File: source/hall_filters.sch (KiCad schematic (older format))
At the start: 5 parts

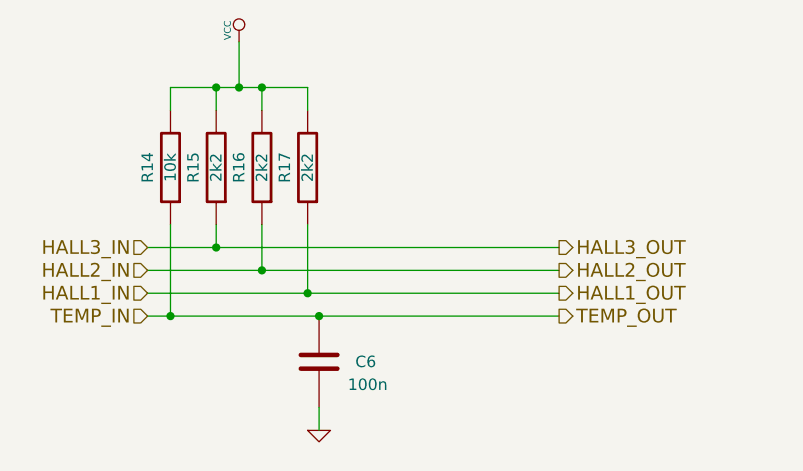
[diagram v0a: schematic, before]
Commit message: V1.0
V1.0
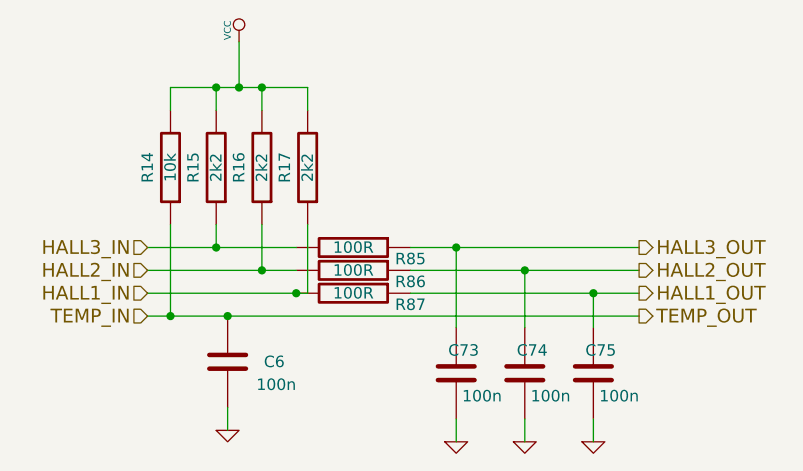
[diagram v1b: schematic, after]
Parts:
- added C73, C74, C75: 100n, Capacitor_SMD:C_0603_1608Metric, symbol BLDC_4-rescue:C-RESCUE-BLDC_4
- added R85, R86, R87: 100R, Resistor_SMD:R_0603_1608Metric, symbol BLDC_4-rescue:R-RESCUE-BLDC_4
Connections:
- net GND: now also C73.1, C74.1, C75.1
- net HALL1_IN: now also R87.2
- net HALL2_IN: now also R86.2
- net HALL3_IN: now also R85.2
- new net HALL1_OUT: C75.2, R87.1
- new net HALL2_OUT: C74.2, R86.1
- new net HALL3_OUT: C73.2, R85.1
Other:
- moved on the sheet: C6
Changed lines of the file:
@@
 Text HLabel 3500 3350 0    60   Input ~ 0
 TEMP_IN
-Text HLabel 5300 3050 2    60   Output ~ 0
+Text HLabel 5650 3050 2    60   Output ~ 0
 HALL3_OUT
-Text HLabel 5300 3150 2    60   Output ~ 0
+Text HLabel 5650 3150 2    60   Output ~ 0
 HALL2_OUT
-Text HLabel 5300 3250 2    60   Output ~ 0
+Text HLabel 5650 3250 2    60   Output ~ 0
 HALL1_OUT
-Text HLabel 5300 3350 2    60   Output ~ 0
+Text HLabel 5650 3350 2    60   Output ~ 0
 TEMP_OUT
 $Comp
 L BLDC_4-rescue:C-RESCUE-BLDC_4 C?
 U 1 1 5C7712C3
-P 4250 3550
+P 3850 3550
 AR Path="/5C7712C3" Ref="C?"  Part="1"
 AR Path="/53FBA77E/5C7712C3" Ref="C6"  Part="1"
-F 0 "C6" H 4000 3550 50  0000 L CNN
-F 1 "100n" H 3950 3650 50  0000 L CNN
-F 2 "Capacitor_SMD:C_0603_1608Metric" H 4250 3550 60  0001 C CNN
-F 3 "" H 4250 3550 60  0001 C CNN
-	1    4250 3550
-	-1   0    0    1
-$EndComp
-Wire Wire Line
-	4250 3350 5300 3350
+F 0 "C6" H 3600 3550 50  0000 L CNN
+F 1 "100n" H 3550 3650 50  0000 L CNN
+F 2 "Capacitor_SMD:C_0603_1608Metric" H 3850 3550 60  0001 C CNN
+F 3 "" H 3850 3550 60  0001 C CNN
+	1    3850 3550
+	-1   0    0    1
+$EndComp
 $Comp
 L BLDC_4-rescue:GND-RESCUE-BLDC_4 #PWR?
 U 1 1 5C7716C9
-P 4250 3850
+P 3850 3850
 AR Path="/504F83BE/5C7716C9" Ref="#PWR?"  Part="1"
 AR Path="/53FBA77E/5C7716C9" Ref="#PWR024"  Part="1"
-F 0 "#PWR024" H 4250 3850 30  0001 C CNN
-F 1 "GND" H 4250 3780 30  0001 C CNN
-F 2 "" H 4250 3850 60  0001 C CNN
-F 3 "" H 4250 3850 60  0001 C CNN
-	1    4250 3850
-	1    0    0    -1
-$EndComp
-Wire Wire Line
-	4250 3750 4250 3850
-Wire Wire Line
-	3600 3350 4250 3350
+F 0 "#PWR024" H 3850 3850 30  0001 C CNN
+F 1 "GND" H 3850 3780 30  0001 C CNN
+F 2 "" H 3850 3850 60  0001 C CNN
+F 3 "" H 3850 3850 60  0001 C CNN
+	1    3850 3850
+	1    0    0    -1
+$EndComp
+Wire Wire Line
+	3850 3750 3850 3850
+Wire Wire Line
+	3600 3350 3850 3350
 Connection ~ 3600 3350
-Connection ~ 4250 3350
-Connection ~ 4200 3250
-Wire Wire Line
-	4200 3250 5300 3250
-Wire Wire Line
-	3500 3250 4200 3250
+Wire Wire Line
+	3500 3250 4150 3250
 Connection ~ 4000 2350
 Wire Wire Line
 	4000 2350 4200 2350
-Connection ~ 4000 3150
-Wire Wire Line
-	4000 3150 5300 3150
 Wire Wire Line
 	3500 3150 4000 3150
@@
 Wire Wire Line
 	3800 2350 3900 2350
-Connection ~ 3800 3050
-Wire Wire Line
-	3800 3050 5300 3050
 Wire Wire Line
 	3500 3050 3800 3050
@@
 Wire Wire Line
 	3900 2350 4000 2350
+$Comp
+L BLDC_4-rescue:R-RESCUE-BLDC_4 R85
+U 1 1 5F21ADDA
+P 4400 3050
+F 0 "R85" V 4450 3300 50  0000 C CNN
+F 1 "100R" V 4400 3050 50  0000 C CNN
+F 2 "Resistor_SMD:R_0603_1608Metric" H 4400 3050 60  0001 C CNN
+F 3 "" H 4400 3050 60  0001 C CNN
+	1    4400 3050
+	0    1    1    0
+$EndComp
+$Comp
+L BLDC_4-rescue:R-RESCUE-BLDC_4 R86
+U 1 1 5F21B279
+P 4400 3150
+F 0 "R86" V 4450 3400 50  0000 C CNN
+F 1 "100R" V 4400 3150 50  0000 C CNN
+F 2 "Resistor_SMD:R_0603_1608Metric" H 4400 3150 60  0001 C CNN
+F 3 "" H 4400 3150 60  0001 C CNN
+	1    4400 3150
+	0    1    1    0
+$EndComp
+$Comp
+L BLDC_4-rescue:R-RESCUE-BLDC_4 R87
+U 1 1 5F21B6A2
+P 4400 3250
+F 0 "R87" V 4450 3500 50  0000 C CNN
+F 1 "100R" V 4400 3250 50  0000 C CNN
+F 2 "Resistor_SMD:R_0603_1608Metric" H 4400 3250 60  0001 C CNN
+F 3 "" H 4400 3250 60  0001 C CNN
+	1    4400 3250
+	0    1    1    0
+$EndComp
+Wire Wire Line
+	4150 3050 3800 3050
+Connection ~ 3800 3050
+Wire Wire Line
+	4000 3150 4150 3150
+Connection ~ 4000 3150
+Wire Wire Line
+	4150 3250 4200 3250
+Connection ~ 4150 3250
+$Comp
+L BLDC_4-rescue:C-RESCUE-BLDC_4 C?
+U 1 1 5F21FBD2
+P 5150 3600
+AR Path="/5F21FBD2" Ref="C?"  Part="1"
+AR Path="/53FBA77E/5F21FBD2" Ref="C74"  Part="1"
+F 0 "C74" H 5050 3500 50  0000 L CNN
+F 1 "100n" H 4950 3700 50  0000 L CNN
+F 2 "Capacitor_SMD:C_0603_1608Metric" H 5150 3600 60  0001 C CNN
+F 3 "" H 5150 3600 60  0001 C CNN
+	1    5150 3600
+	-1   0    0    1
+$EndComp
+$Comp
+L BLDC_4-rescue:GND-RESCUE-BLDC_4 #PWR?
+U 1 1 5F21FBD8
+P 5150 3900
+AR Path="/504F83BE/5F21FBD8" Ref="#PWR?"  Part="1"
+AR Path="/53FBA77E/5F21FBD8" Ref="#PWR054"  Part="1"
+F 0 "#PWR054" H 5150 3900 30  0001 C CNN
+F 1 "GND" H 5150 3830 30  0001 C CNN
+F 2 "" H 5150 3900 60  0001 C CNN
+F 3 "" H 5150 3900 60  0001 C CNN
+	1    5150 3900
+	1    0    0    -1
+$EndComp
+Wire Wire Line
+	5150 3800 5150 3900
+Connection ~ 3850 3350
+Wire Wire Line
+	3850 3350 5650 3350
+Wire Wire Line
+	4650 3250 5450 3250
+Wire Wire Line
+	4850 3800 4850 3900
+$Comp
+L BLDC_4-rescue:GND-RESCUE-BLDC_4 #PWR?
+U 1 1 5F21F69A
+P 4850 3900
+AR Path="/504F83BE/5F21F69A" Ref="#PWR?"  Part="1"
+AR Path="/53FBA77E/5F21F69A" Ref="#PWR043"  Part="1"
+F 0 "#PWR043" H 4850 3900 30  0001 C CNN
+F 1 "GND" H 4850 3830 30  0001 C CNN
+F 2 "" H 4850 3900 60  0001 C CNN
+F 3 "" H 4850 3900 60  0001 C CNN
+	1    4850 3900
+	1    0    0    -1
+$EndComp
+$Comp
+L BLDC_4-rescue:C-RESCUE-BLDC_4 C?
+U 1 1 5F21F694
+P 4850 3600
+AR Path="/5F21F694" Ref="C?"  Part="1"
+AR Path="/53FBA77E/5F21F694" Ref="C73"  Part="1"
+F 0 "C73" H 4750 3500 50  0000 L CNN
+F 1 "100n" H 4650 3700 50  0000 L CNN
+F 2 "Capacitor_SMD:C_0603_1608Metric" H 4850 3600 60  0001 C CNN
+F 3 "" H 4850 3600 60  0001 C CNN
+	1    4850 3600
+	-1   0    0    1
+$EndComp
+$Comp
+L BLDC_4-rescue:C-RESCUE-BLDC_4 C?
+U 1 1 5F222283
+P 5450 3600
+AR Path="/5F222283" Ref="C?"  Part="1"
+AR Path="/53FBA77E/5F222283" Ref="C75"  Part="1"
+F 0 "C75" H 5350 3500 50  0000 L CNN
+F 1 "100n" H 5250 3700 50  0000 L CNN
+F 2 "Capacitor_SMD:C_0603_1608Metric" H 5450 3600 60  0001 C CNN
+F 3 "" H 5450 3600 60  0001 C CNN
+	1    5450 3600
+	-1   0    0    1
+$EndComp
+$Comp
+L BLDC_4-rescue:GND-RESCUE-BLDC_4 #PWR?
+U 1 1 5F222289
+P 5450 3900
+AR Path="/504F83BE/5F222289" Ref="#PWR?"  Part="1"
+AR Path="/53FBA77E/5F222289" Ref="#PWR088"  Part="1"
+F 0 "#PWR088" H 5450 3900 30  0001 C CNN
+F 1 "GND" H 5450 3830 30  0001 C CNN
+F 2 "" H 5450 3900 60  0001 C CNN
+F 3 "" H 5450 3900 60  0001 C CNN
+	1    5450 3900
+	1    0    0    -1
+$EndComp
+Wire Wire Line
+	5450 3800 5450 3900
+Wire Wire Line
+	4850 3400 4850 3050
+Wire Wire Line
+	5150 3400 5150 3150
+Wire Wire Line
+	5450 3400 5450 3250
+Connection ~ 5450 3250
+Wire Wire Line
+	5450 3250 5650 3250
+Connection ~ 4850 3050
+Wire Wire Line
+	4850 3050 5650 3050
+Connection ~ 5150 3150
+Wire Wire Line
+	5150 3150 5650 3150
+Wire Wire Line
+	4650 3150 5150 3150
+Wire Wire Line
+	4650 3050 4850 3050
 $EndSCHEMATC
